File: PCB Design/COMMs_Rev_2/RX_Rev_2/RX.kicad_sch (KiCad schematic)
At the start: 51 parts, among them J1 Conn_01x24_Pin, J2 Conn_01x24_Pin, J3 Conn_01x03_Pin, J4 Conn_01x04_Pin, J5 Conn_01x02_Pin, U1 TLV9101IDCKR, U2 TPD2E007DCKR, U3 INA828IDR, U4 OPA2322AIDGKR

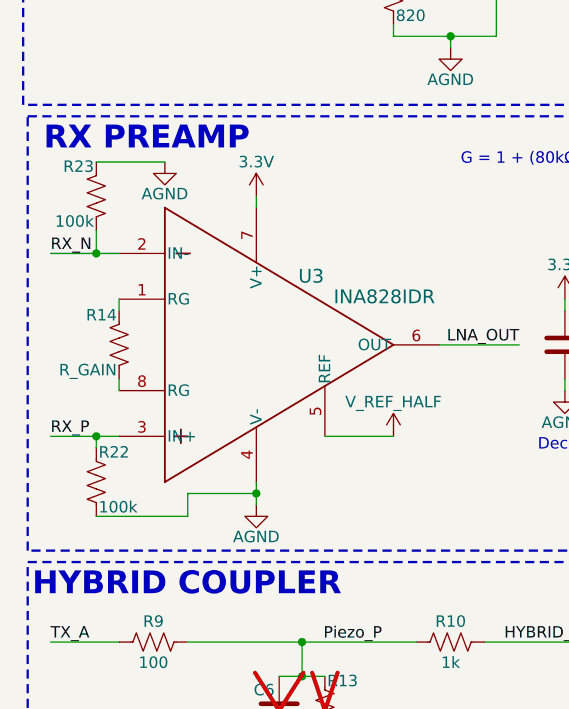
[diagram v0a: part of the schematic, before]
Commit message: Updated
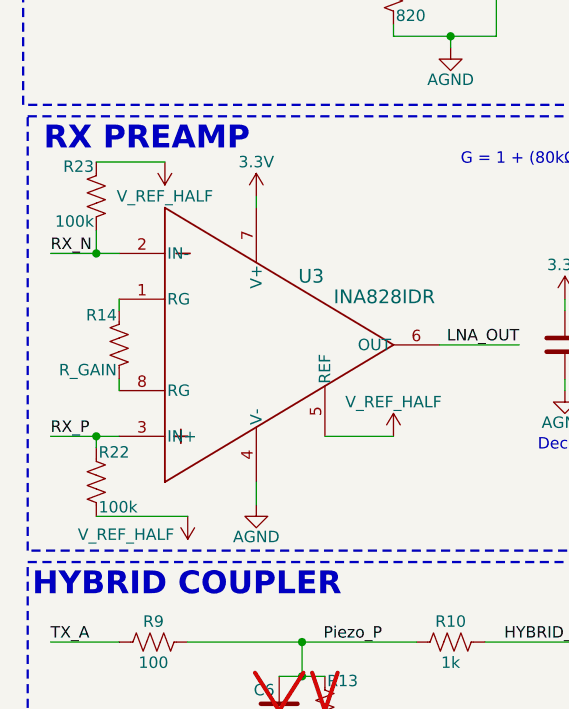
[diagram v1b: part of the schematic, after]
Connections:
- net AGND: no longer R22.2, R23.1
- net V_REF_HALF: now also R22.2, R23.1
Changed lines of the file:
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@@
 	)
 	(junction
-		(at 39.37 137.16)
-		(diameter 0)
-		(color 0 0 0 0)
-	)
-	(junction
 		(at 64.77 69.85)
 		(diameter 0)
@@
 	(wire
 		(pts
-			(xy 39.37 135.89) (xy 39.37 137.16)
+			(xy 39.37 135.89) (xy 39.37 138.43)
 		)
 		(stroke
@@
 	(wire
 		(pts
-			(xy 31.75 137.16) (xy 39.37 137.16)
-		)
-		(stroke
-			(width 0)
-			(type default)
-		)
-	)
-	(wire
-		(pts
 			(xy 45.72 35.56) (xy 45.72 43.18)
 		)
@@
 	(wire
 		(pts
-			(xy 39.37 137.16) (xy 39.37 138.43)
-		)
-		(stroke
-			(width 0)
-			(type default)
-		)
-	)
-	(wire
-		(pts
 			(xy 153.67 20.32) (xy 162.56 20.32)
 		)
@@
 	(wire
 		(pts
-			(xy 31.75 139.7) (xy 31.75 137.16)
-		)
-		(stroke
-			(width 0)
-			(type default)
-		)
-	)
-	(wire
-		(pts
 			(xy 275.59 88.9) (xy 275.59 85.09)
 		)
@@
 	)
 	(symbol
-		(lib_id "power:GND")
-		(at 29.21 100.33 0)
-		(unit 1)
-		(body_style 1)
-		(exclude_from_sim no)
-		(in_bom yes)
-		(on_board yes)
-		(in_pos_files yes)
-		(dnp no)
-		(property "Reference" "#PWR037"
-			(at 29.21 106.68 0)
-			(hide yes)
-			(show_name no)
-			(do_not_autoplace no)
-			(effects
-				(font
-					(size 1.27 1.27)
-				)
-			)
-		)
-		(property "Value" "AGND"
-			(at 29.21 103.886 0)
-			(show_name no)
-			(do_not_autoplace no)
-			(effects
-				(font
-					(size 1.27 1.27)
-				)
-			)
-		)
-		(property "Footprint" ""
-			(at 29.21 100.33 0)
-			(hide yes)
-			(show_name no)
-			(do_not_autoplace no)
-			(effects
-				(font
-					(size 1.27 1.27)
-				)
-			)
-		)
-		(property "Datasheet" ""
-			(at 29.21 100.33 0)
-			(hide yes)
-			(show_name no)
-			(do_not_autoplace no)
-			(effects
-				(font
-					(size 1.27 1.27)
-				)
-			)
-		)
-		(property "Description" "Power symbol creates a global label with name \"GND\" , ground"
-			(at 29.21 100.33 0)
-			(hide yes)
-			(show_name no)
-			(do_not_autoplace no)
-			(effects
-				(font
-					(size 1.27 1.27)
-				)
-			)
-		)
-		(pin "1"
-		)
-		(instances
-			(project "RX"
-				(path "/487393bf-b13e-4fd8-b19d-84bece8bafcd"
-					(reference "#PWR037")
-					(unit 1)
-				)
-			)
-		)
-	)
-	(symbol
 		(lib_id "power:VCC")
 		(at 240.03 21.59 270)
@@
 	)
 	(symbol
+		(lib_id "power:VCC")
+		(at 31.75 139.7 180)
+		(unit 1)
+		(body_style 1)
+		(exclude_from_sim no)
+		(in_bom yes)
+		(on_board yes)
+		(in_pos_files yes)
+		(dnp no)
+		(property "Reference" "#PWR038"
+			(at 31.75 135.89 0)
+			(hide yes)
+			(show_name no)
+			(do_not_autoplace no)
+			(effects
+				(font
+					(size 1.27 1.27)
+				)
+			)
+		)
+		(property "Value" "V_REF_HALF"
+			(at 24.892 141.732 0)
+			(show_name no)
+			(do_not_autoplace no)
+			(effects
+				(font
+					(size 1.27 1.27)
+				)
+			)
+		)
+		(property "Footprint" ""
+			(at 31.75 139.7 0)
+			(hide yes)
+			(show_name no)
+			(do_not_autoplace no)
+			(effects
+				(font
+					(size 1.27 1.27)
+				)
+			)
+		)
+		(property "Datasheet" ""
+			(at 31.75 139.7 0)
+			(hide yes)
+			(show_name no)
+			(do_not_autoplace no)
+			(effects
+				(font
+					(size 1.27 1.27)
+				)
+			)
+		)
+		(property "Description" "Power symbol creates a global label with name \"VCC\""
+			(at 31.75 139.7 0)
+			(hide yes)
+			(show_name no)
+			(do_not_autoplace no)
+			(effects
+				(font
+					(size 1.27 1.27)
+				)
+			)
+		)
+		(pin "1"
+		)
+		(instances
+			(project "RX"
+				(path "/487393bf-b13e-4fd8-b19d-84bece8bafcd"
+					(reference "#PWR038")
+					(unit 1)
+				)
+			)
+		)
+	)
+	(symbol
 		(lib_id "Device:R_US")
 		(at 110.49 72.39 90)
@@
 					(unit 1)
 				)
+			)
+		)
+	)
+	(symbol
+		(lib_id "power:VCC")
+		(at 29.21 100.33 180)
+		(unit 1)
+		(body_style 1)
+		(exclude_from_sim no)
+		(in_bom yes)
+		(on_board yes)
+		(in_pos_files yes)
+		(dnp no)
+		(property "Reference" "#PWR037"
+			(at 29.21 96.52 0)
+			(hide yes)
+			(show_name no)
+			(do_not_autoplace no)
+			(effects
+				(font
+					(size 1.27 1.27)
+				)
+			)
+		)
+		(property "Value" "V_REF_HALF"
+			(at 29.21 104.14 0)
+			(show_name no)
+			(do_not_autoplace no)
+			(effects
+				(font
+					(size 1.27 1.27)
+				)
+			)
+		)
+		(property "Footprint" ""
+			(at 29.21 100.33 0)
+			(hide yes)
+			(show_name no)
+			(do_not_autoplace no)
+			(effects
+				(font
+					(size 1.27 1.27)
+				)
+			)
+		)
+		(property "Datasheet" ""
+			(at 29.21 100.33 0)
+			(hide yes)
+			(show_name no)
+			(do_not_autoplace no)
+			(effects
+				(font
+					(size 1.27 1.27)
+				)
+			)
+		)
+		(property "Description" "Power symbol creates a global label with name \"VCC\""
+			(at 29.21 100.33 0)
+			(hide yes)
+			(show_name no)
+			(do_not_autoplace no)
+			(effects
+				(font
+					(size 1.27 1.27)
+				)
+			)
+		)
+		(pin "1"
+		)
+		(instances
+			(project "RX"
+				(path "/487393bf-b13e-4fd8-b19d-84bece8bafcd"
+					(reference "#PWR037")
+					(unit 1)
+				)

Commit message: Revert "Updated"
This reverts commit 89be44ed720659141c8ee702c54a520a60db740f.
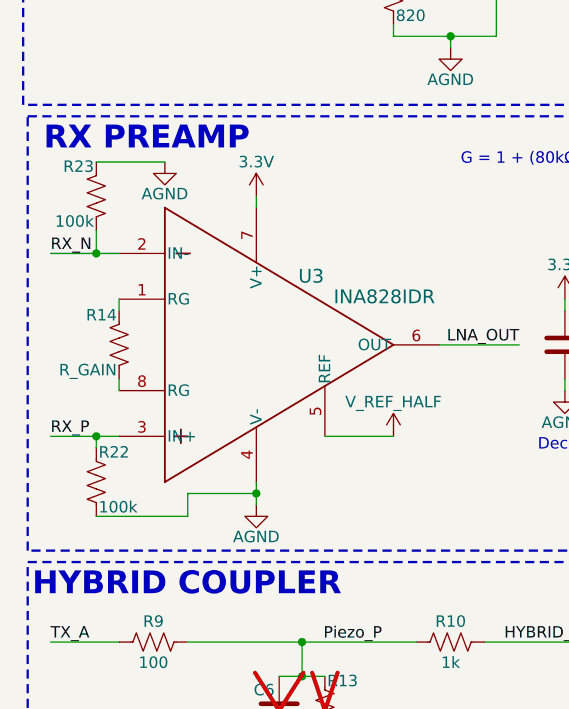
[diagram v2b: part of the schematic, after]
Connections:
- net AGND: now also R22.2, R23.1
- net V_REF_HALF: no longer R22.2, R23.1
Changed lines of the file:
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@@
 	)
 	(junction
+		(at 39.37 137.16)
+		(diameter 0)
+		(color 0 0 0 0)
+	)
+	(junction
 		(at 64.77 69.85)
 		(diameter 0)
@@
 	(wire
 		(pts
-			(xy 39.37 135.89) (xy 39.37 138.43)
+			(xy 39.37 135.89) (xy 39.37 137.16)
 		)
 		(stroke
@@
 	(wire
 		(pts
+			(xy 31.75 137.16) (xy 39.37 137.16)
+		)
+		(stroke
+			(width 0)
+			(type default)
+		)
+	)
+	(wire
+		(pts
 			(xy 45.72 35.56) (xy 45.72 43.18)
 		)
@@
 	(wire
 		(pts
+			(xy 39.37 137.16) (xy 39.37 138.43)
+		)
+		(stroke
+			(width 0)
+			(type default)
+		)
+	)
+	(wire
+		(pts
 			(xy 153.67 20.32) (xy 162.56 20.32)
 		)
@@
 	(wire
 		(pts
+			(xy 31.75 139.7) (xy 31.75 137.16)
+		)
+		(stroke
+			(width 0)
+			(type default)
+		)
+	)
+	(wire
+		(pts
 			(xy 275.59 88.9) (xy 275.59 85.09)
 		)
@@
 	)
 	(symbol
+		(lib_id "power:GND")
+		(at 29.21 100.33 0)
+		(unit 1)
+		(body_style 1)
+		(exclude_from_sim no)
+		(in_bom yes)
+		(on_board yes)
+		(in_pos_files yes)
+		(dnp no)
+		(property "Reference" "#PWR037"
+			(at 29.21 106.68 0)
+			(hide yes)
+			(show_name no)
+			(do_not_autoplace no)
+			(effects
+				(font
+					(size 1.27 1.27)
+				)
+			)
+		)
+		(property "Value" "AGND"
+			(at 29.21 103.886 0)
+			(show_name no)
+			(do_not_autoplace no)
+			(effects
+				(font
+					(size 1.27 1.27)
+				)
+			)
+		)
+		(property "Footprint" ""
+			(at 29.21 100.33 0)
+			(hide yes)
+			(show_name no)
+			(do_not_autoplace no)
+			(effects
+				(font
+					(size 1.27 1.27)
+				)
+			)
+		)
+		(property "Datasheet" ""
+			(at 29.21 100.33 0)
+			(hide yes)
+			(show_name no)
+			(do_not_autoplace no)
+			(effects
+				(font
+					(size 1.27 1.27)
+				)
+			)
+		)
+		(property "Description" "Power symbol creates a global label with name \"GND\" , ground"
+			(at 29.21 100.33 0)
+			(hide yes)
+			(show_name no)
+			(do_not_autoplace no)
+			(effects
+				(font
+					(size 1.27 1.27)
+				)
+			)
+		)
+		(pin "1"
+		)
+		(instances
+			(project "RX"
+				(path "/487393bf-b13e-4fd8-b19d-84bece8bafcd"
+					(reference "#PWR037")
+					(unit 1)
+				)
+			)
+		)
+	)
+	(symbol
 		(lib_id "power:VCC")
 		(at 240.03 21.59 270)
@@
 	)
 	(symbol
-		(lib_id "power:VCC")
-		(at 31.75 139.7 180)
-		(unit 1)
-		(body_style 1)
-		(exclude_from_sim no)
-		(in_bom yes)
-		(on_board yes)
-		(in_pos_files yes)
-		(dnp no)
-		(property "Reference" "#PWR038"
-			(at 31.75 135.89 0)
-			(hide yes)
-			(show_name no)
-			(do_not_autoplace no)
-			(effects
-				(font
-					(size 1.27 1.27)
-				)
-			)
-		)
-		(property "Value" "V_REF_HALF"
-			(at 24.892 141.732 0)
-			(show_name no)
-			(do_not_autoplace no)
-			(effects
-				(font
-					(size 1.27 1.27)
-				)
-			)
-		)
-		(property "Footprint" ""
-			(at 31.75 139.7 0)
-			(hide yes)
-			(show_name no)
-			(do_not_autoplace no)
-			(effects
-				(font
-					(size 1.27 1.27)
-				)
-			)
-		)
-		(property "Datasheet" ""
-			(at 31.75 139.7 0)
-			(hide yes)
-			(show_name no)
-			(do_not_autoplace no)
-			(effects
-				(font
-					(size 1.27 1.27)
-				)
-			)
-		)
-		(property "Description" "Power symbol creates a global label with name \"VCC\""
-			(at 31.75 139.7 0)
-			(hide yes)
-			(show_name no)
-			(do_not_autoplace no)
-			(effects
-				(font
-					(size 1.27 1.27)
-				)
-			)
-		)
-		(pin "1"
-		)
-		(instances
-			(project "RX"
-				(path "/487393bf-b13e-4fd8-b19d-84bece8bafcd"
-					(reference "#PWR038")
-					(unit 1)
-				)
-			)
-		)
-	)
-	(symbol
 		(lib_id "Device:R_US")
 		(at 110.49 72.39 90)
@@
 					(unit 1)
 				)
-			)
-		)
-	)
-	(symbol
-		(lib_id "power:VCC")
-		(at 29.21 100.33 180)
-		(unit 1)
-		(body_style 1)
-		(exclude_from_sim no)
-		(in_bom yes)
-		(on_board yes)
-		(in_pos_files yes)
-		(dnp no)
-		(property "Reference" "#PWR037"
-			(at 29.21 96.52 0)
-			(hide yes)
-			(show_name no)
-			(do_not_autoplace no)
-			(effects
-				(font
-					(size 1.27 1.27)
-				)
-			)
-		)
-		(property "Value" "V_REF_HALF"
-			(at 29.21 104.14 0)
-			(show_name no)
-			(do_not_autoplace no)
-			(effects
-				(font
-					(size 1.27 1.27)
-				)
-			)
-		)
-		(property "Footprint" ""
-			(at 29.21 100.33 0)
-			(hide yes)
-			(show_name no)
-			(do_not_autoplace no)
-			(effects
-				(font
-					(size 1.27 1.27)
-				)
-			)
-		)
-		(property "Datasheet" ""
-			(at 29.21 100.33 0)
-			(hide yes)
-			(show_name no)
-			(do_not_autoplace no)
-			(effects
-				(font
-					(size 1.27 1.27)
-				)
-			)
-		)
-		(property "Description" "Power symbol creates a global label with name \"VCC\""
-			(at 29.21 100.33 0)
-			(hide yes)
-			(show_name no)
-			(do_not_autoplace no)
-			(effects
-				(font
-					(size 1.27 1.27)
-				)
-			)
-		)
-		(pin "1"
-		)
-		(instances
-			(project "RX"
-				(path "/487393bf-b13e-4fd8-b19d-84bece8bafcd"
-					(reference "#PWR037")
-					(unit 1)
-				)
